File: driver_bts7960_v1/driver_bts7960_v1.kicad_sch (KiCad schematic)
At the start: 28 parts, among them J1 Motor_1, J2 Alimentacion, J3 Conn_02x04_Odd_Even, J6 Motor_2, U1 BTS7960B, U2 BTS7960B, U3 BTS7960B, U4 BTS7960B, U5 74HC244

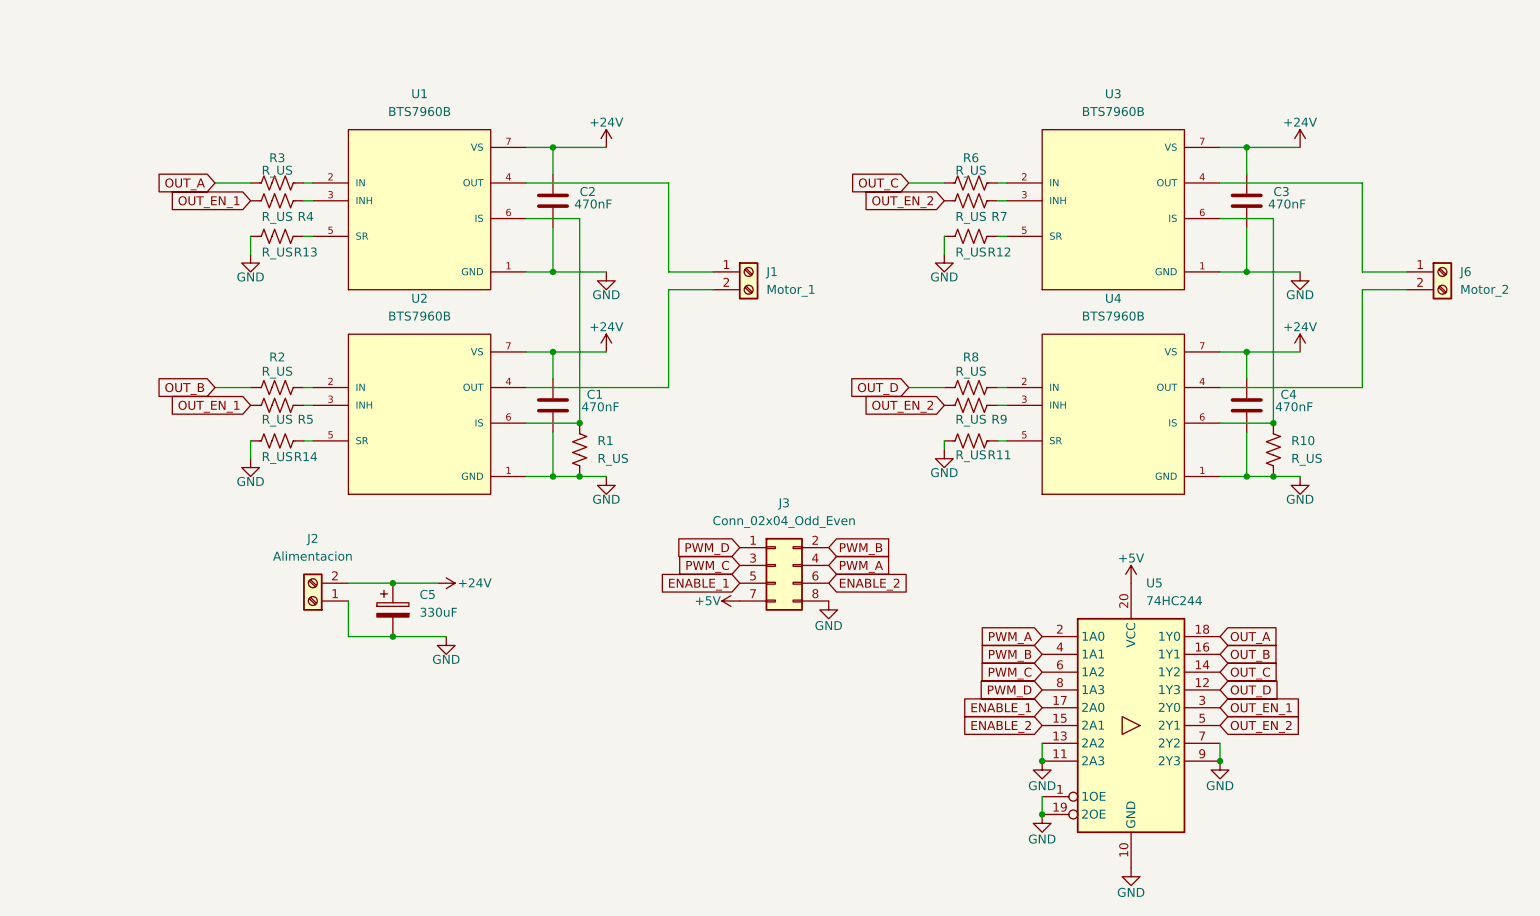
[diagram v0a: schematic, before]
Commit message: .
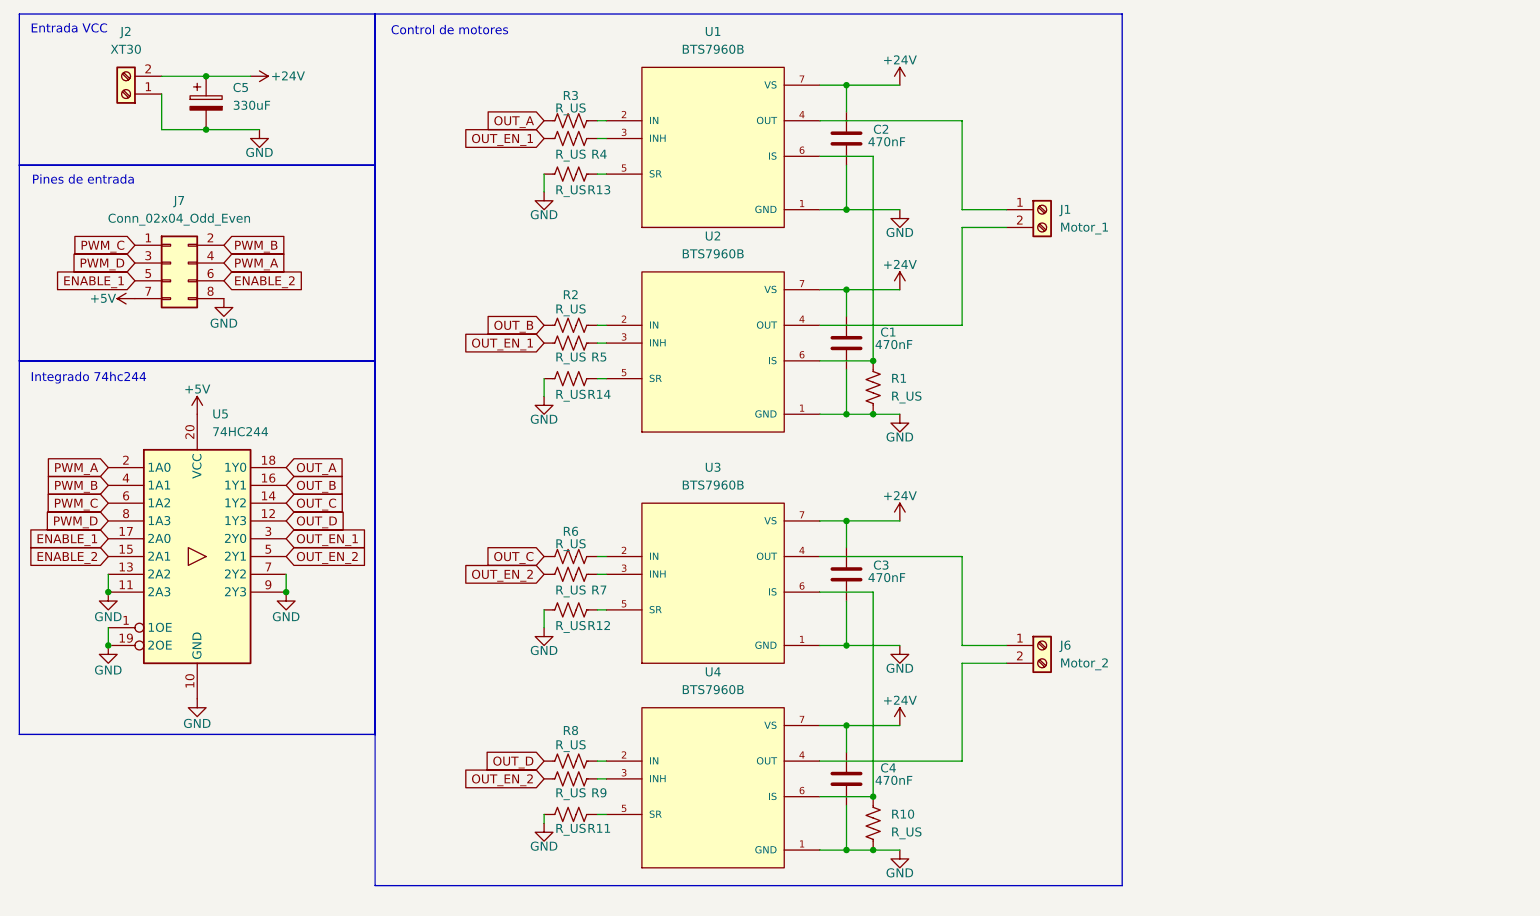
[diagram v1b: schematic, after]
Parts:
- removed J3: Conn_02x04_Odd_Even, Connector_PinHeader_2.54mm:PinHeader_2x04_P2.54mm_Vertical, symbol Connector_Generic:Conn_02x04_Odd_Even
- added J7: Conn_02x04_Odd_Even, Connector_PinHeader_2.54mm:PinHeader_2x04_P2.54mm_Vertical, symbol Connector_Generic:Conn_02x04_Odd_Even
- C5: footprint Capacitor_THT:CP_Radial_D10.0mm_P5.00mm -> Capacitor_THT:CP_Radial_D8.0mm_P3.80mm
- J2: value Alimentacion -> XT30; footprint Connector_AMASS:AMASS_XT30UPB-F_1x02_P5.0mm_Vertical -> Connector_AMASS:AMASS_XT30U-F_1x02_P5.0mm_Vertical
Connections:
- net +5V: now also J7.7 (Pin_7)
- net ENABLE_1: now also J7.5 (Pin_5)
- net ENABLE_2: now also J7.6 (Pin_6)
- net GND: now also J7.8 (Pin_8)
- net PWM_A: now also J7.4 (Pin_4)
- net PWM_B: now also J7.2 (Pin_2)
- net PWM_C: now also J7.1 (Pin_1)
- net PWM_D: now also J7.3 (Pin_3)
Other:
- note added: "Control de motores"
- note added: "Entrada VCC"
- note added: "Integrado 74hc244"
- note added: "Pines de entrada"
- moved on the sheet: C1, C2, C3, C4, C5, J1, J2, J6, R1, R10, R11, R12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
